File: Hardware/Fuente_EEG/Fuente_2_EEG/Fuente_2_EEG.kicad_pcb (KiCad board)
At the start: 2 copper layers, 56 x 29 mm, 24 parts, among them J1 Mounting_Hole, J3 Power_Jack, J4 Power_BAT, J5 Vout_opAmp, J6 Vout_uC, SW1 SW_DIP, U1 ICL7660

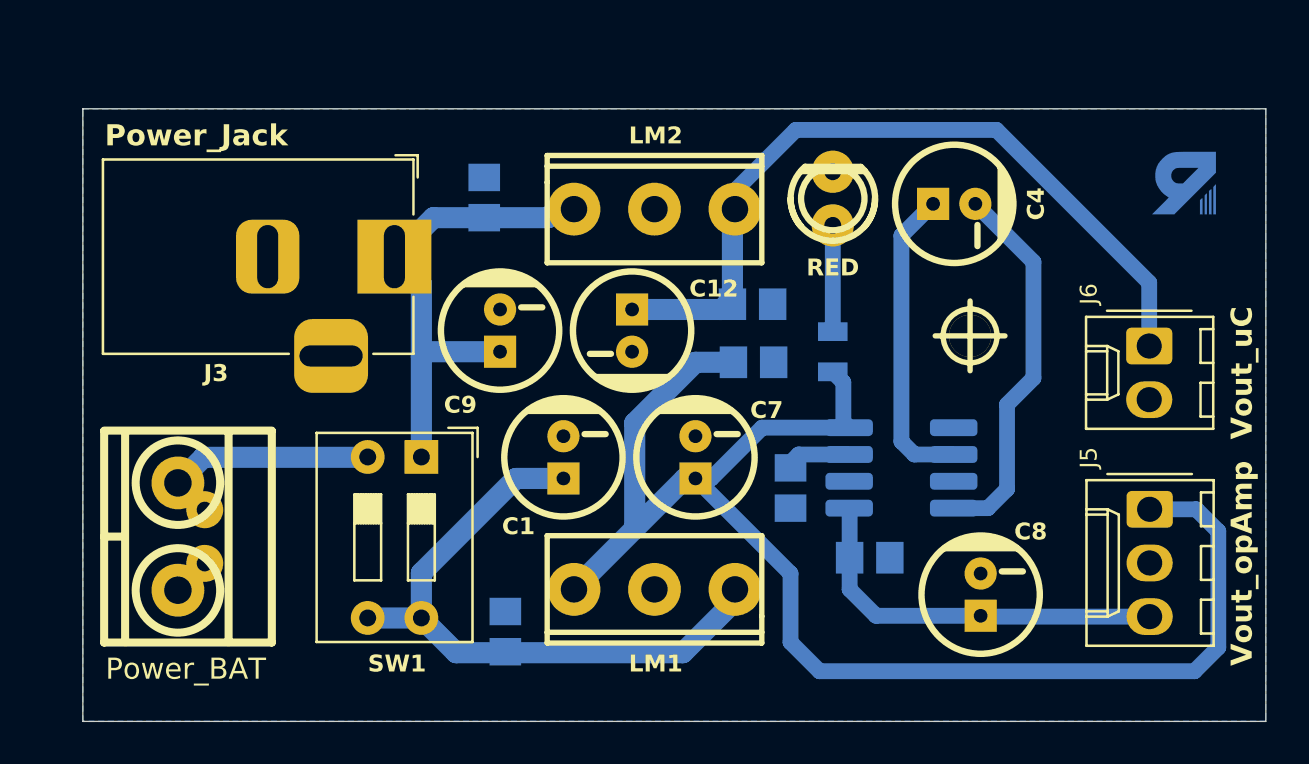
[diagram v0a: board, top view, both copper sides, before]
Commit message: Add files via upload
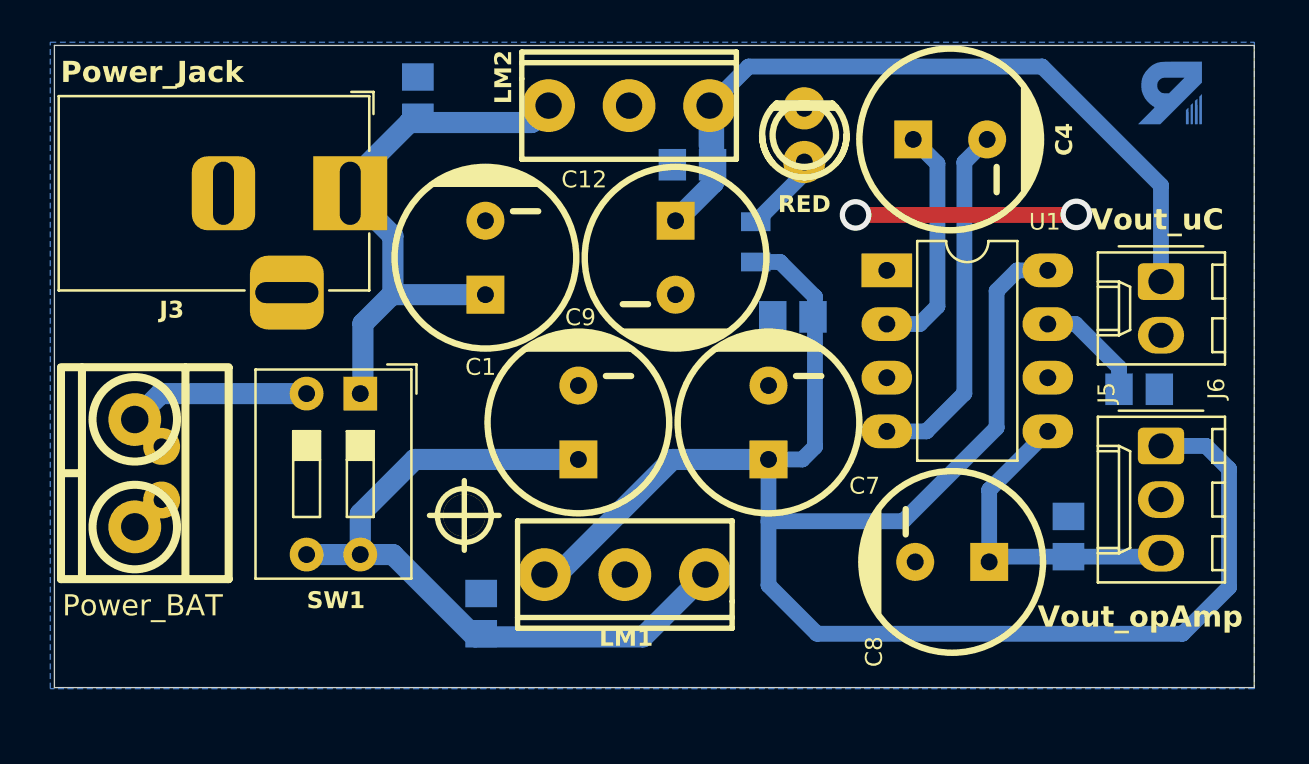
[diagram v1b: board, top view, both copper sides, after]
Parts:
- C1, C12, C4, C7, C8, C9: footprint EESTN5:CAP_ELEC_5x11mm -> EESTN5:CAP_ELEC_8x11.5mm
- U1: footprint Package_SO:SOIC-8_3.9x4.9mm_P1.27mm -> EESTN5:DIP-8; moved to F.Cu
- moved J1 25.4 mm to (144.7, 109.0)
- moved C2 17.2 mm to (176.6, 103.0), turned to 180 degrees
- moved C6 9.46 mm to (173.3, 110.0), turned to -90 degrees
- moved U1 9.38 mm to (164.7, 97.4), turned to 0 degrees
- moved C11 7.19 mm to (155.5, 92.4), turned to 0 degrees
- moved R1 6.35 mm to (158.4, 96.0)
- moved C10 5.70 mm to (142.5, 89.2)
- moved LM2 5.05 mm to (152.5, 89.6)
- moved G*** 4.32 mm to (178.1, 89.0)
- moved SW1 4.17 mm to (139.7, 103.2)
- moved C12 4.02 mm to (154.7, 96.8)
- moved C7 3.83 mm to (159.1, 104.6)
- moved J3 3.66 mm to (139.3, 93.8)
- moved J4 3.63 mm to (129.1, 107.0)
- moved C9 3.52 mm to (145.7, 96.8)
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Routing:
- net +5V: track 70.3 -> 86.7 mm
- net GND: track 0.00 -> 10.5 mm, vias 0 -> 2
- net VCC: track 30.3 -> 35.0 mm
- net +9V: track 22.8 -> 26.9 mm
- net -5V: track 18.6 -> 15.4 mm
- net Net-(U1-CAP+): track 14.6 -> 11.6 mm
- net Net-(U1-OSC): track 3.18 -> 5.27 mm
- net Net-(LED1-A): track 5.03 -> 3.78 mm
- net Net-(U1-CAP-): track 18.1 -> 16.9 mm
- net +7.5V: track 9.49 -> 8.64 mm
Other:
- board size 56 x 29 mm -> 56.8 x 30.4 mm
